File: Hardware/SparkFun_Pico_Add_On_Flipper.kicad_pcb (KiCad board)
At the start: 2 copper layers, 25.4 x 50.8 mm, 109 parts, among them J1 Conn_01x20, J2 Conn_01x20, J3 Conn_01x20, J4 Conn_01x20, J5 Qwiic_RA, SW1 SMD_RA_5x3mm_h3.6mm

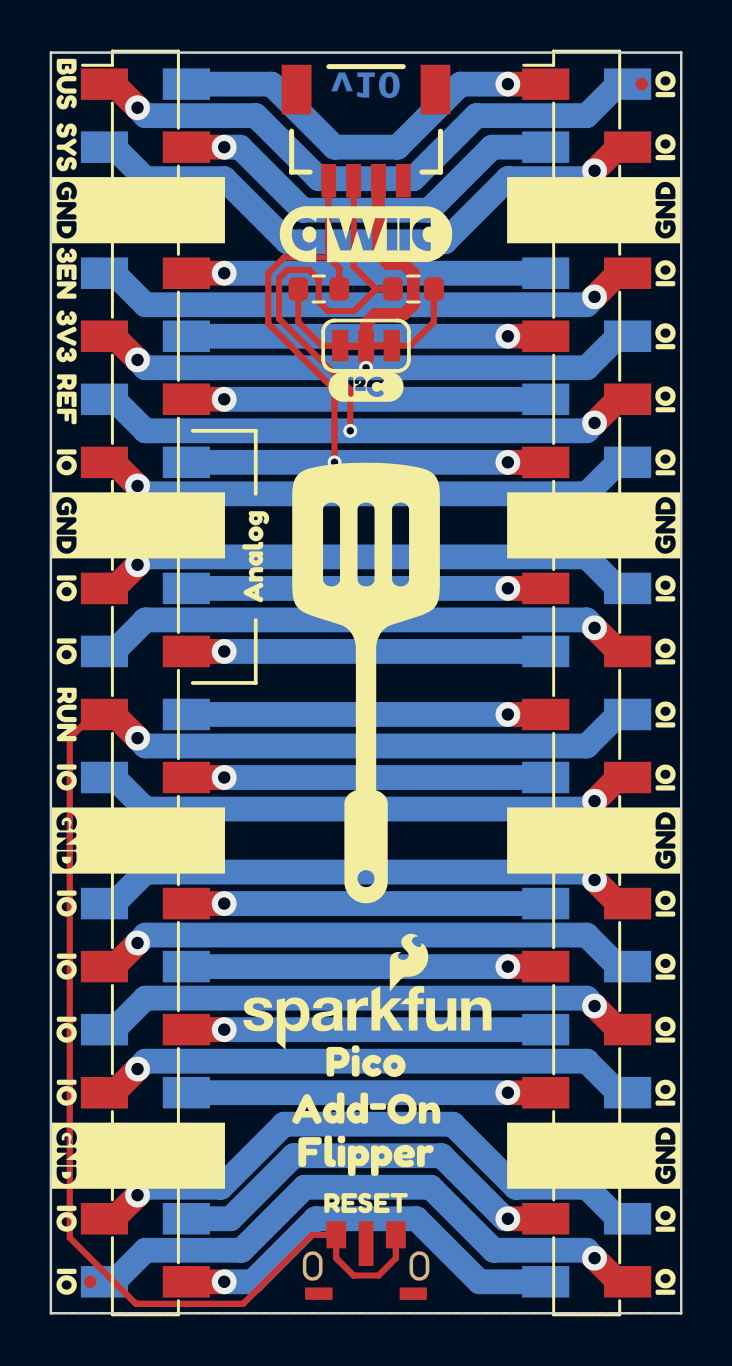
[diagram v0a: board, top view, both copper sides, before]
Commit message: Tweak routing
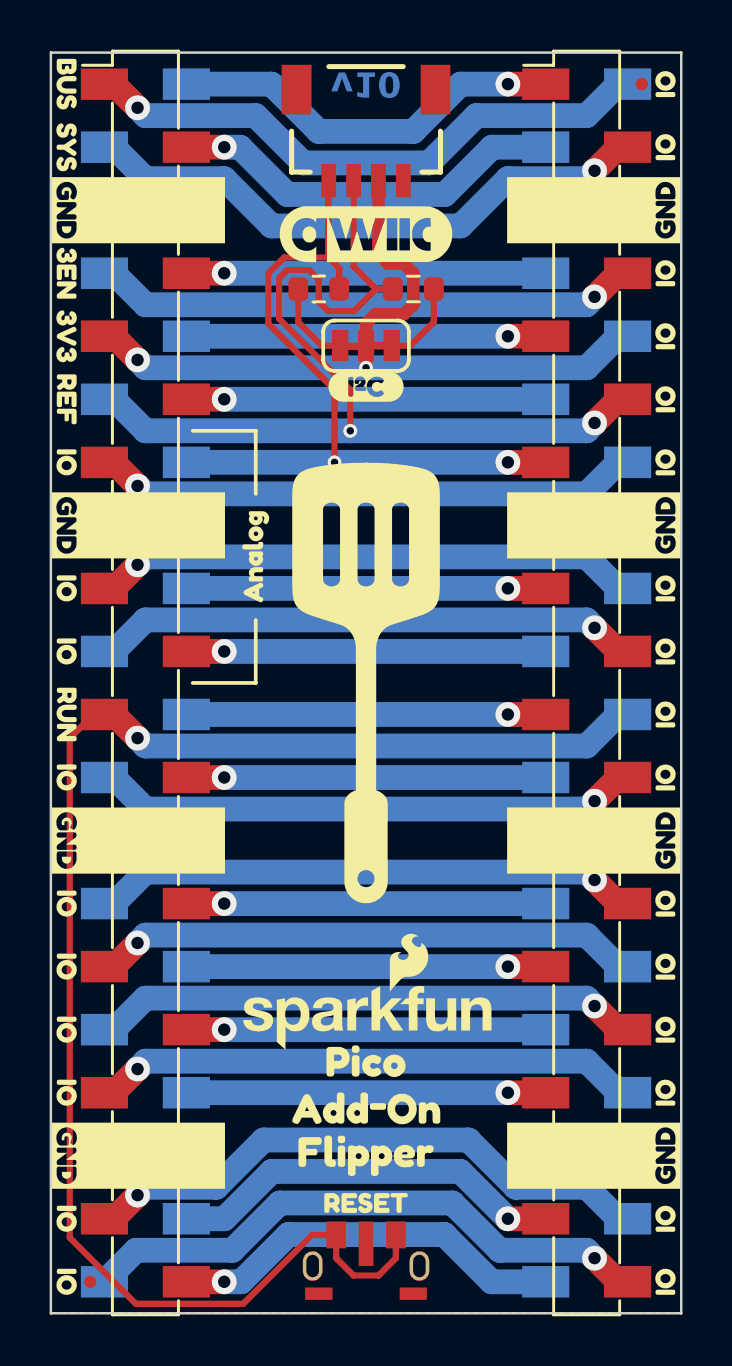
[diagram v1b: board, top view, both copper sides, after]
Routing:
- net IO15: track 24.2 -> 23.7 mm
- net VSYS: track 16.6 -> 16.1 mm
- net IO14: track 16.6 -> 16.1 mm
- net IO0: track 16.6 -> 16.1 mm
- net IO1: track 24.2 -> 23.7 mm
- net VBUS: track 24.2 -> 23.7 mm
- net IO17: track 24.2 -> 23.7 mm
- net IO16: track 16.6 -> 16.1 mm
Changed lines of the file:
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@@
 	)
 	(segment
-		(start 133.985 78.74)
-		(end 131.445 81.28)
+		(start 137.16 78.74)
+		(end 133.985 78.74)
 		(width 1)
 		(layer "B.Cu")
@@
 	)
 	(segment
-		(start 125.095 81.28)
+		(start 122.555 78.74)
+		(end 119.38 78.74)
+		(width 1)
+		(layer "B.Cu")
+		(net 14)
+	)
+	(segment
+		(start 133.985 78.74)
+		(end 132.08 80.645)
+		(width 1)
+		(layer "B.Cu")
+		(net 14)
+	)
+	(segment
+		(start 132.08 80.645)
+		(end 124.46 80.645)
+		(width 1)
+		(layer "B.Cu")
+		(net 14)
+	)
+	(segment
+		(start 124.46 80.645)
 		(end 122.555 78.74)
 		(width 1)
@@
 	)
 	(segment
-		(start 137.16 78.74)
-		(end 133.985 78.74)
-		(width 1)
-		(layer "B.Cu")
-		(net 14)
-	)
-	(segment
-		(start 122.555 78.74)
-		(end 119.38 78.74)
-		(width 1)
-		(layer "B.Cu")
-		(net 14)
-	)
-	(segment
 		(start 118.11 77.47)
 		(end 117.73 77.47)
@@
 	)
 	(segment
-		(start 131.445 81.28)
-		(end 125.095 81.28)
-		(width 1)
-		(layer "B.Cu")
-		(net 14)
-	)
-	(segment
 		(start 138.43 102.87)
 		(end 138.81 102.87)
@@
 	)
 	(segment
-		(start 127 77.47)
-		(end 124.46 74.93)
+		(start 124.46 74.93)
+		(end 121.03 74.93)
 		(width 1)
 		(layer "B.Cu")
@@
 	)
 	(segment
+		(start 130.175 76.835)
+		(end 126.365 76.835)
+		(width 1)
+		(layer "B.Cu")
+		(net 18)
+	)
+	(segment
 		(start 132.08 74.93)
-		(end 129.54 77.47)
+		(end 130.175 76.835)
 		(width 1)
 		(layer "B.Cu")
@@
 	)
 	(segment
-		(start 124.46 74.93)
-		(end 121.03 74.93)
-		(width 1)
-		(layer "B.Cu")
-		(net 18)
-	)
-	(segment
-		(start 129.54 77.47)
-		(end 127 77.47)
+		(start 126.365 76.835)
+		(end 124.46 74.93)
 		(width 1)
 		(layer "B.Cu")
@@
 	)
 	(segment
-		(start 126.238 120.65)
-		(end 130.302 120.65)
+		(start 123.237625 123.19)
+		(end 125.142625 121.285)
 		(width 1)
 		(layer "B.Cu")
@@
 	)
 	(segment
-		(start 130.302 120.65)
-		(end 132.842 123.19)
+		(start 131.426046 121.285)
+		(end 133.331046 123.19)
 		(width 1)
 		(layer "B.Cu")
@@
 	)
 	(segment
+		(start 125.142625 121.285)
+		(end 131.426046 121.285)
+		(width 1)
+		(layer "B.Cu")
+		(net 22)
+	)
+	(segment
 		(start 122.555 123.19)
-		(end 123.698 123.19)
+		(end 123.237625 123.19)
 		(width 1)
 		(layer "B.Cu")
@@
 	)
 	(segment
-		(start 132.842 123.19)
+		(start 133.331046 123.19)
 		(end 135.51 123.19)
-		(width 1)
-		(layer "B.Cu")
-		(net 22)
-	)
-	(segment
-		(start 123.698 123.19)
-		(end 126.238 120.65)
 		(width 1)
 		(layer "B.Cu")
@@
 	)
 	(segment
-		(start 130.175 78.74)
+		(start 123.825 76.2)
+		(end 125.73 78.105)
+		(width 1)
+		(layer "B.Cu")
+		(net 28)
+	)
+	(segment
+		(start 138.43 74.93)
+		(end 138.81 74.93)
+		(width 1)
+		(layer "B.Cu")
+		(net 28)
+	)
+	(segment
+		(start 130.81 78.105)
 		(end 132.715 76.2)
+		(width 1)
+		(layer "B.Cu")
+		(net 28)
+	)
+	(segment
+		(start 119.0625 75.8825)
+		(end 119.38 76.2)
 		(width 1)
 		(layer "B.Cu")
@@
 	)
 	(segment
-		(start 119.0625 75.8825)
-		(end 119.38 76.2)
+		(start 125.73 78.105)
+		(end 130.81 78.105)
+		(width 1)
+		(layer "B.Cu")
+		(net 28)
+	)
+	(segment
+		(start 132.715 76.2)
+		(end 137.16 76.2)
 		(width 1)
 		(layer "B.Cu")
@@
 	)
 	(segment
-		(start 132.715 76.2)
-		(end 137.16 76.2)
-		(width 1)
-		(layer "B.Cu")
-		(net 28)
-	)
-	(segment
-		(start 123.825 76.2)
-		(end 126.365 78.74)
-		(width 1)
-		(layer "B.Cu")
-		(net 28)
-	)
-	(segment
-		(start 126.365 78.74)
-		(end 130.175 78.74)
-		(width 1)
-		(layer "B.Cu")
-		(net 28)
-	)
-	(segment
-		(start 138.43 74.93)
-		(end 138.81 74.93)
-		(width 1)
-		(layer "B.Cu")
-		(net 28)
-	)
-	(segment
 		(start 118.11 120.65)
 		(end 117.73 120.65)
@@
 	)
 	(segment
-		(start 122.428 119.38)
-		(end 124.968 116.84)
+		(start 132.3975 117.475)
+		(end 134.3025 119.38)
+		(width 1)
+		(layer "B.Cu")
+		(net 29)
+	)
+	(segment
+		(start 119.0625 119.6975)
+		(end 119.38 119.38)
+		(width 1)
+		(layer "B.Cu")
+		(net 29)
+	)
+	(segment
+		(start 124.1425 117.475)
+		(end 132.3975 117.475)
+		(width 1)
+		(layer "B.Cu")
+		(net 29)
+	)
+	(segment
+		(start 119.38 119.38)
+		(end 122.2375 119.38)
+		(width 1)
+		(layer "B.Cu")
+		(net 29)
+	)
+	(segment
+		(start 138.43 120.65)
+		(end 138.81 120.65)
+		(width 1)
+		(layer "B.Cu")
+		(net 29)
+	)
+	(segment
+		(start 122.2375 119.38)
+		(end 124.1425 117.475)
 		(width 1)
 		(layer "B.Cu")
@@
 	)
 	(segment
-		(start 119.38 119.38)
-		(end 122.428 119.38)
-		(width 1)
-		(layer "B.Cu")
-		(net 29)
-	)
-	(segment
-		(start 124.968 116.84)
-		(end 131.7625 116.84)
-		(width 1)
-		(layer "B.Cu")
-		(net 29)
-	)
-	(segment
-		(start 119.0625 119.6975)
-		(end 119.38 119.38)
-		(width 1)
-		(layer "B.Cu")
-		(net 29)
-	)
-	(segment
-		(start 131.7625 116.84)
-		(end 134.3025 119.38)
-		(width 1)
-		(layer "B.Cu")
-		(net 29)
-	)
-	(segment
-		(start 138.43 120.65)
-		(end 138.81 120.65)
-		(width 1)
-		(layer "B.Cu")
-		(net 29)
-	)
-	(segment
 		(start 119.0625 109.5375)
 		(end 118.11 110.49)
@@
 	(segment
 		(start 133.35 77.47)
-		(end 130.81 80.01)
+		(end 131.445 79.375)
+		(width 1)
+		(layer "B.Cu")
+		(net 32)
+	)
+	(segment
+		(start 131.445 79.375)
+		(end 125.095 79.375)
+		(width 1)
+		(layer "B.Cu")
+		(net 32)
+	)
+	(segment
+		(start 125.095 79.375)
+		(end 123.19 77.47)
 		(width 1)
 		(layer "B.Cu")
@@
 	)
 	(segment
-		(start 130.81 80.01)
-		(end 125.73 80.01)
-		(width 1)
-		(layer "B.Cu")
-		(net 32)
-	)
-	(segment
-		(start 125.73 80.01)
-		(end 123.19 77.47)
-		(width 1)
-		(layer "B.Cu")
-		(net 32)
-	)
-	(segment
 		(start 118.11 90.17)
 		(end 117.73 90.17)
@@
 	)
 	(segment
-		(start 122.809 120.65)
-		(end 125.349 118.11)
+		(start 124.466318 118.745)
+		(end 132.073682 118.745)
 		(width 1)
 		(layer "B.Cu")
@@
 	)
 	(segment
-		(start 133.858 120.65)
+		(start 133.978682 120.65)
 		(end 133.985 120.65)
 		(width 1)
@@
 	)
 	(segment
-		(start 125.349 118.11)
-		(end 131.318 118.11)
+		(start 122.561318 120.65)
+		(end 124.466318 118.745)
 		(width 1)
 		(layer "B.Cu")
@@
 	(segment
 		(start 121.03 120.65)
-		(end 122.809 120.65)
+		(end 122.561318 120.65)
 		(width 1)
 		(layer "B.Cu")
@@
 	)
 	(segment
-		(start 131.318 118.11)
-		(end 133.858 120.65)
+		(start 132.073682 118.745)
+		(end 133.978682 120.65)
 		(width 1)
 		(layer "B.Cu")
@@
 	)
 	(segment
-		(start 125.7935 119.38)
-		(end 123.2535 121.92)
+		(start 137.16 121.92)
+		(end 133.654864 121.92)
 		(width 1)
 		(layer "B.Cu")
@@
 	)
 	(segment
-		(start 137.16 121.92)
-		(end 133.4135 121.92)
+		(start 133.654864 121.92)
+		(end 131.749864 120.015)
 		(width 1)
 		(layer "B.Cu")
@@
 	)
 	(segment
-		(start 119.38 121.92)
-		(end 118.11 123.19)
+		(start 122.885136 121.92)
+		(end 119 121.92)
 		(width 1)
 		(layer "B.Cu")
@@
 	)
 	(segment
-		(start 123.2535 121.92)
-		(end 119.38 121.92)
-		(width 1)
-		(layer "B.Cu")
-		(net 37)
-	)
-	(segment
-		(start 130.8735 119.38)
-		(end 125.7935 119.38)
-		(width 1)
-		(layer "B.Cu")
-		(net 37)
-	)
-	(segment
-		(start 133.4135 121.92)
-		(end 130.8735 119.38)
+		(start 119 121.92)
+		(end 117.73 123.19)
 		(width 1)
 		(layer "B.Cu")
@@
 	)
 	(segment
-		(start 118.11 123.19)
-		(end 117.73 123.19)
-		(width 1)
-		(layer "B.Cu")
+		(start 131.749864 120.015)
+		(end 124.790136 120.015)
+		(width 1)
+		(layer "B.Cu")
+		(net 37)
+	)
+	(segment
+		(start 124.790136 120.015)
+		(end 122.885136 121.92)
+		(width 1)
+		(layer "B.Cu")
